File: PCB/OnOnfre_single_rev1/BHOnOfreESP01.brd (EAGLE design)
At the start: 53 x 55 mm, 25 parts, among them K1 OMRON-G3MB-202P-SSR2, K2 OMRON-G3MB-202P-SSR2, Q1 S8050, Q2 S8050, SW1 B3U-1000P-2P-SMD, SW2 B3U-1000P-2P-SMD

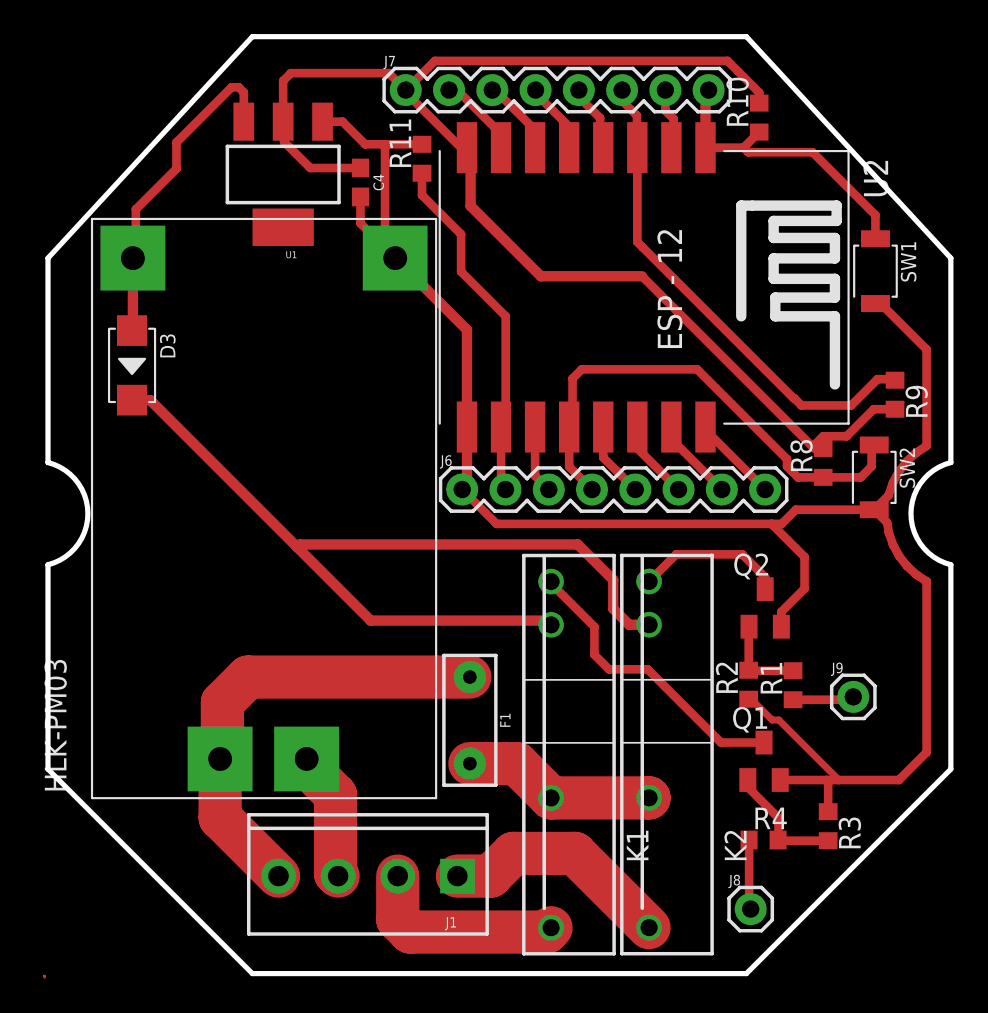
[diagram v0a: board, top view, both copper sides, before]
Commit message: Organização do repositorio
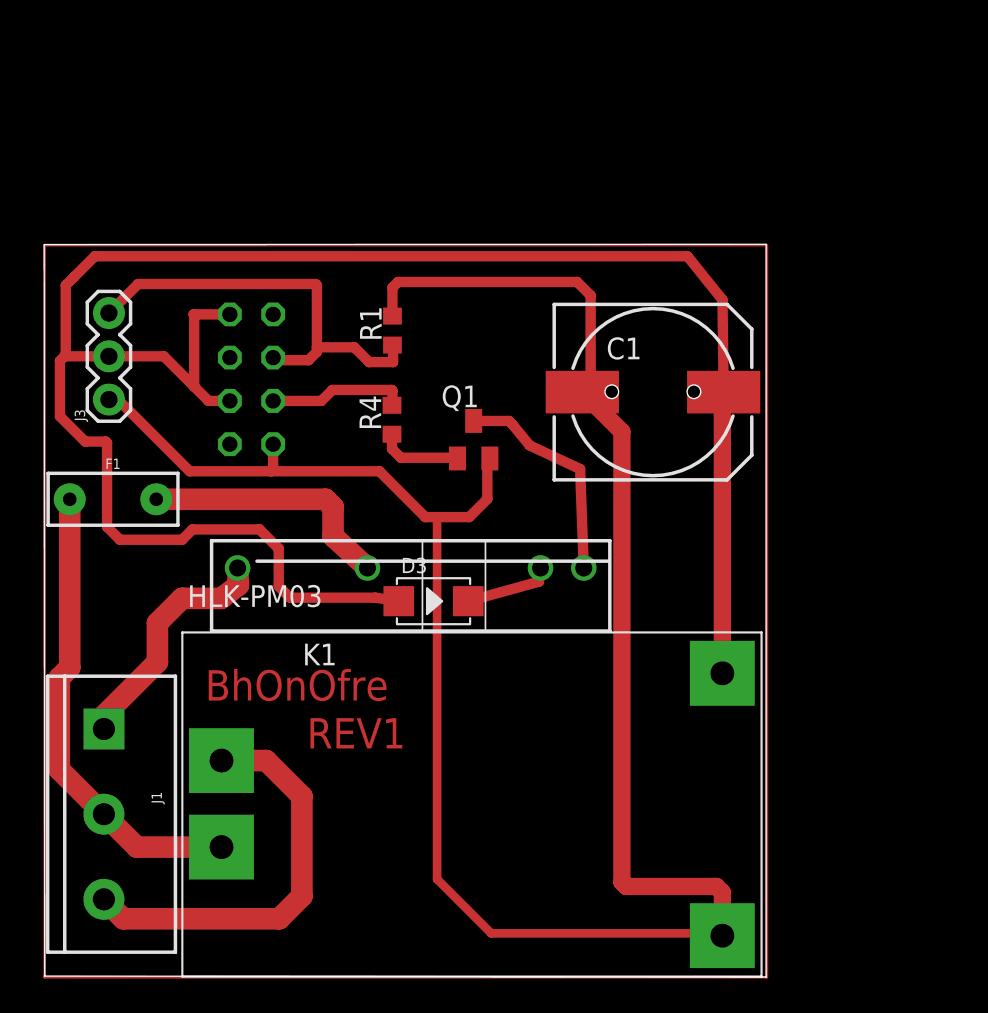
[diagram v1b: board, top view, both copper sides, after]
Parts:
- removed C4: 100nF, SparkFun-Capacitors:0603
- removed J6, J7: (no value), SparkFun-Connectors:1X08
- removed J8, J9: (no value), SparkFun-Connectors:1X01
- removed K2: OMRON-G3MB-202P-SSR2, Omron G3MB 202p SSR:OMRON-G3MB-202P-SSR
- removed Q2: S8050, semicon-smd-ipc:SOT23
- removed R10, R11, R2, R3, R8, R9: 10k, resistor:R0603
- removed SW1, SW2: B3U-1000P-2P-SMD, Seeed-Switch:SW2-2.6-3.0X2.5X1.2+0.4MM
- removed U1: (no value), SparkFun-IC-Power:SOT223
- removed U2: (no value), esp8266modules:ESP12-SMD
- added C1: 1000uf, adafruit:140CLH-1010
- added J3: (no value), SparkFun-Connectors:1X03
- added U$3: ESP8266-01, captain-slow:ESP8266-01
- J1: device SparkFun-Connectors:SCREWTERMINAL-3.5MM-4 -> SparkFun-Connectors:SCREWTERMINAL-5MM-3
- R1, R4: value 10k -> 47k
- moved R4 32.9 mm to (20.4, 32.7), turned to 90 degrees
- moved R1 31.4 mm to (20.4, 37.9)
- moved Q1 25.4 mm to (25.2, 31.5)
- moved F1 24.6 mm to (4.01, 28.0), turned to 0 degrees
- moved J1 22.5 mm to (3.48, 14.5), turned to 270 degrees
- moved D3 22.5 mm to (22.8, 22.0), turned to 0 degrees
- moved K1 10.2 mm to (24.0, 24.0), turned to 0 degrees
- moved U$2 7.19 mm to (10.4, 7.57), turned to 0 degrees
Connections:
- removed net 3V3: C4.1, J7.1, R10.2, R8.2, R9.2, U1.2, U2.VCC
- removed net ADC: J7.7, U2.ADC
- removed net CH_PD: J7.6, R9.1, U2.CH_PD
- removed net FASE: J1.3, U$2.AC2
- removed net GPIO0: J6.4, R8.1, SW2.1, U2.GPIO0
- removed net GPIO02: J6.3, U2.GPIO2
- removed net GPIO04: J6.6, U2.GPIO4
- removed net GPIO05: J6.5, U2.GPIO5
- removed net GPIO12: J7.3, U2.GPIO12
- removed net GPIO13: J7.2, U2.GPIO13
- removed net GPIO14: J7.4, U2.GPIO14
- removed net GPIO15: J6.2, R11.1, U2.GPIO15
- removed net GPIO16: J7.5, U2.GPIO16
- removed net N$13: Q2.1, R1.2, R2.2
- removed net NEUTRAL_IN: F1.P$1, J1.4, U$2.AC1
- removed net NEUTRAL_IN_FUSED: F1.P$2, K1.2, K2.2
- removed net NEUTRAL_ONE_OUT: J1.2, K1.1
- removed net NEUTRAL_TWO_OUT: J1.1, K2.1
- removed net R1: J8.1, R4.1
- removed net R2: J9.1, R1.1
- removed net RESET: J7.8, R10.1, SW1.1, U2.RESET
- removed net RX: J6.7, U2.RXD0
- removed net TX: J6.8, U2.TXD0
- new net CH1: R4.2, U$3.GPIO2
- new net N$4: F1.P$1, J1.2, U$2.AC2
- new net N$5: J1.3, U$2.AC1
- new net N$8: D3.2, K1.3
- new net TOUCH: J3.3, R1.1, U$3.GPIO0
- net GND: now also C1.-, J3.1, R1.2, U$3.GND; no longer C4.2, J6.1, Q2.2, R11.2, R2.1, R3.1, SW1.2, SW2.2, U1.1, U2.GND
- net N$2: now also J1.1, K1.1; no longer D3.2, K1.3, K2.3
- net N$7: now also F1.P$2, K1.2; no longer Q1.1, R3.2, R4.2
- net N$9: now also Q1.1, R4.1; no longer K2.4, Q2.3
- net VCC: now also C1.+, J3.2, U$3.3V3, U$3.CH_PD; no longer U1.3
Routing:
- net N$3: track 0.00 -> 170.6 mm
- net VCC: track 19.3 -> 116.9 mm
- net 3V3: track 80.7 -> 0.00 mm
- net N$2: track 53.7 -> 14.2 mm
- net GPIO0: track 29.4 -> 0.00 mm
- net CH_PD: track 29.1 -> 0.00 mm
- net N$4: track 0.11 -> 27.9 mm
- net NEUTRAL_IN: track 26.8 -> 0.00 mm
- net TOUCH: track 0.00 -> 25.5 mm
- net N$5: track 0.00 -> 24.1 mm
- net GPIO15: track 21.0 -> 0.00 mm
- net RESET: track 18.0 -> 0.00 mm
- net NEUTRAL_TWO_OUT: track 13.6 -> 0.00 mm
- net NEUTRAL_ONE_OUT: track 12.0 -> 0.00 mm
- net NEUTRAL_IN_FUSED: track 11.4 -> 0.00 mm
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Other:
- board size 53 x 55 mm -> 42.4 x 43 mm
- board text added: "BhOnOfre"
- board text added: "REV1"
